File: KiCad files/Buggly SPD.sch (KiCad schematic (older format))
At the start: 6 parts, among them J1 Conn_01x07, J2 Conn_01x05, J3 Conn_01x08, J4 Conn_01x02, J5 Conn_02x03_Odd_Even, J6 Conn_01x02

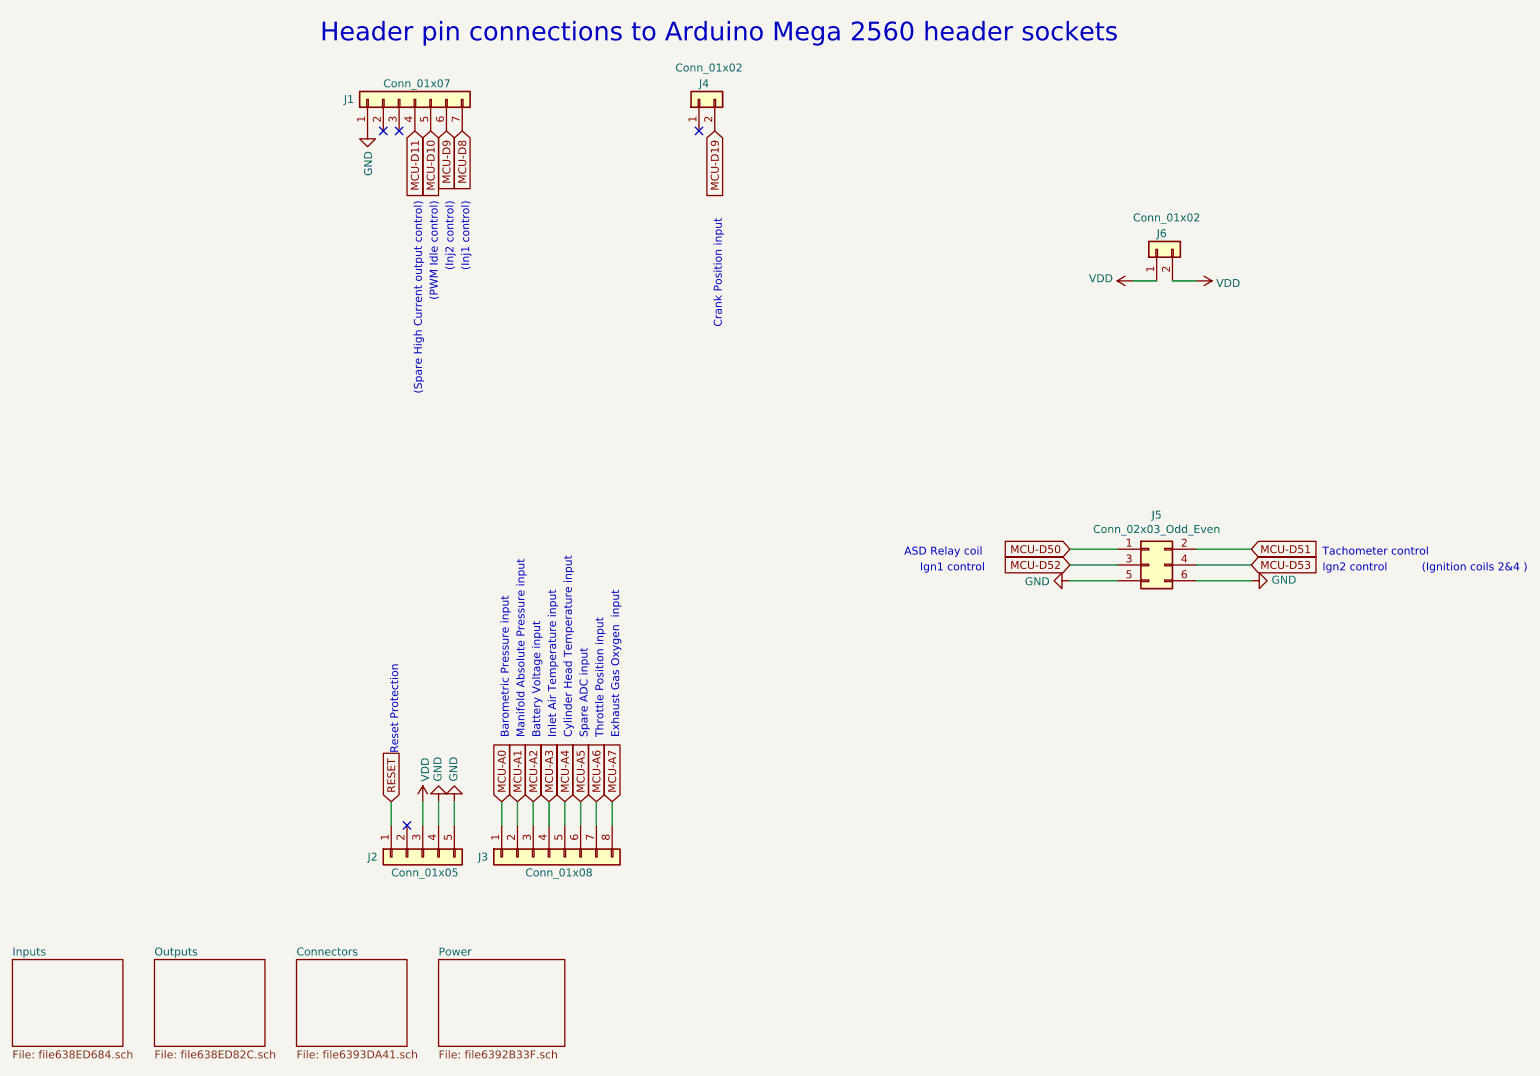
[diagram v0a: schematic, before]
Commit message: Add files via upload
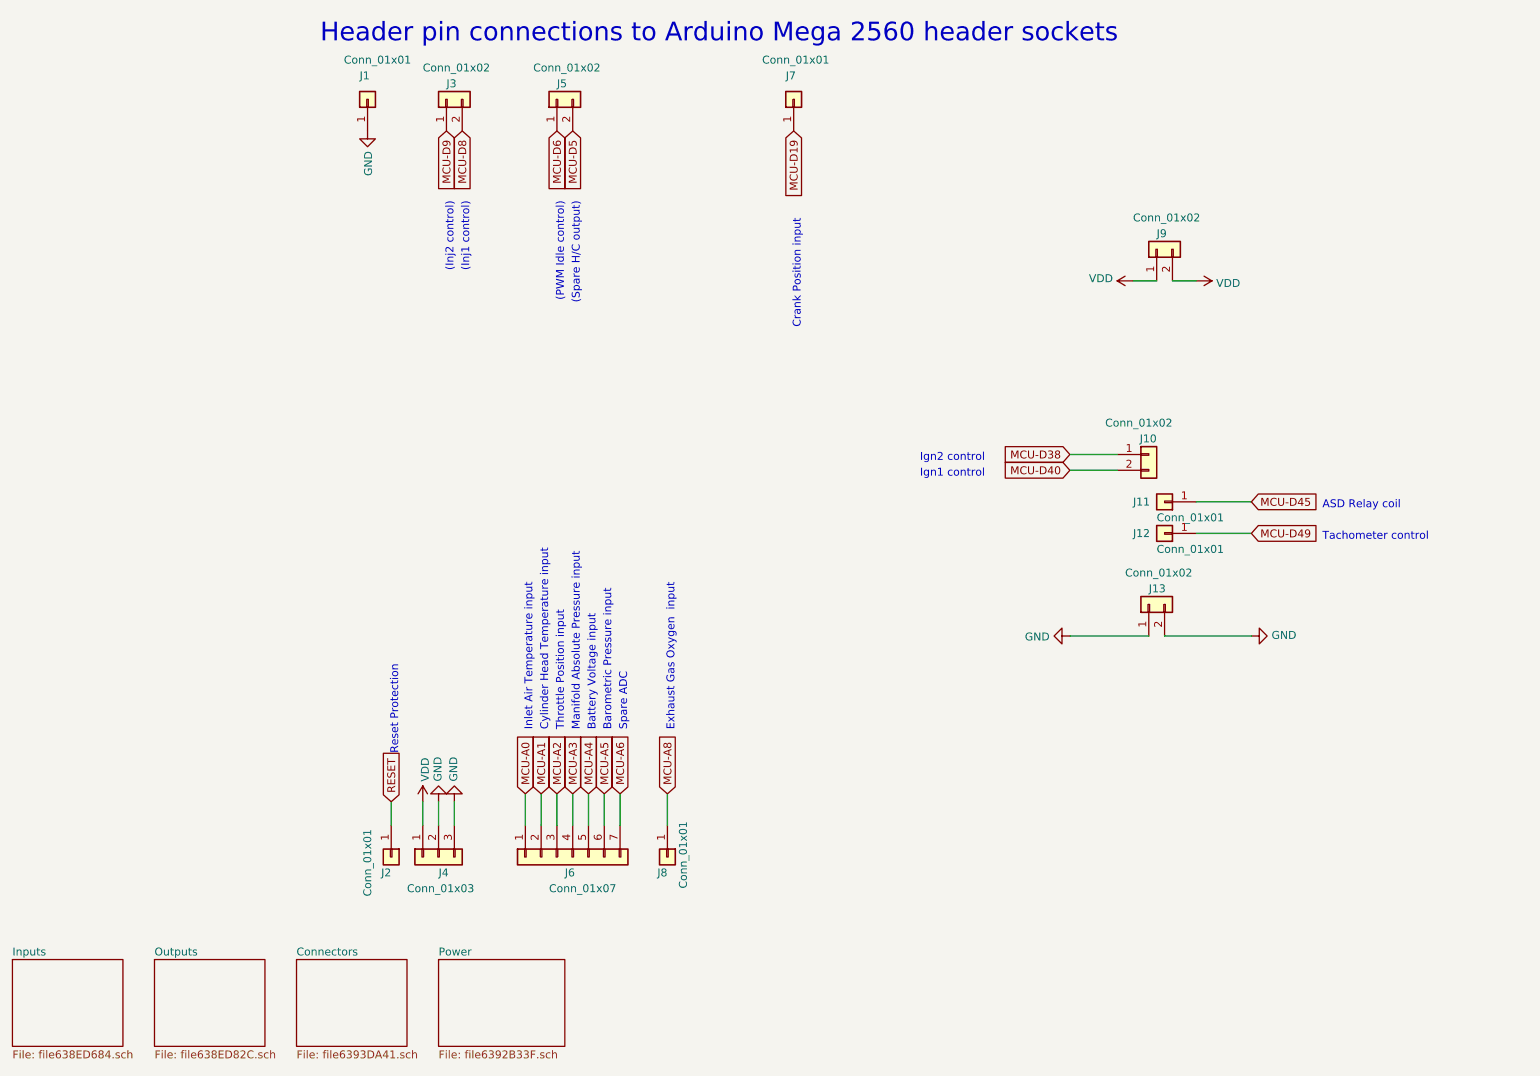
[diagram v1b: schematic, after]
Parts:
- removed J1: Conn_01x07, Connector_PinHeader_2.54mm:PinHeader_1x07_P2.54mm_Vertical, symbol Connector_Generic:Conn_01x07
- removed J2: Conn_01x05, Connector_PinHeader_2.54mm:PinHeader_1x05_P2.54mm_Vertical, symbol Connector_Generic:Conn_01x05
- removed J3: Conn_01x08, Connector_PinHeader_2.54mm:PinHeader_1x08_P2.54mm_Vertical, symbol Connector_Generic:Conn_01x08
- removed J4: Conn_01x02, Connector_PinHeader_2.54mm:PinHeader_1x02_P2.54mm_Vertical, symbol Connector_Generic:Conn_01x02
- removed J5: Conn_02x03_Odd_Even, Connector_PinHeader_2.54mm:PinHeader_2x03_P2.54mm_Vertical, symbol Connector_Generic:Conn_02x03_Odd_Even
- added J1, J11, J12, J2, J7, J8: Conn_01x01, Connector_PinHeader_2.54mm:PinHeader_1x01_P2.54mm_Vertical, symbol Connector_Generic:Conn_01x01
- added J10, J13, J3, J5: Conn_01x02, Connector_PinHeader_2.54mm:PinHeader_1x02_P2.54mm_Vertical, symbol Connector_Generic:Conn_01x02
- added J4: Conn_01x03, Connector_PinHeader_2.54mm:PinHeader_1x03_P2.54mm_Vertical, symbol Connector_Generic:Conn_01x03
- added J6: Conn_01x07, Connector_PinHeader_2.54mm:PinHeader_1x07_P2.54mm_Vertical, symbol Connector_Generic:Conn_01x07
- renumbered J6 to J9
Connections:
- net GND: now also J1.1 (Pin_1), J13.1 (Pin_1), J13.2 (Pin_2), J4.2 (Pin_2), J4.3 (Pin_3)
- net MCU-A0: now also J6.1 (Pin_1)
- net MCU-A1: now also J6.2 (Pin_2)
- net MCU-A2: now also J6.3 (Pin_3)
- net MCU-A3: now also J6.4 (Pin_4)
- net MCU-A4: now also J6.5 (Pin_5)
- net MCU-A5: now also J6.6 (Pin_6)
- net MCU-A6: now also J6.7 (Pin_7)
- net MCU-D19: now also J7.1 (Pin_1)
- net MCU-D8: now also J3.2 (Pin_2)
- net MCU-D9: now also J3.1 (Pin_1)
- net RESET: now also J2.1 (Pin_1)
- net VDD: now also J4.1 (Pin_1)
- new net MCU-A8: J8.1 (Pin_1)
- new net MCU-D38: J10.1 (Pin_1)
- new net MCU-D40: J10.2 (Pin_2)
- new net MCU-D45: J11.1 (Pin_1)
- new net MCU-D49: J12.1 (Pin_1)
- new net MCU-D5: J5.2 (Pin_2)
- new net MCU-D6: J5.1 (Pin_1)
- no-connect marks 4 -> 0
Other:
- note added: "(Spare H/C output)"
- note added: "Spare ADC"
- note removed: "(Ignition coils 2&4 )"
- note removed: "(Spare High Current output control)"
- note removed: "Spare ADC input"

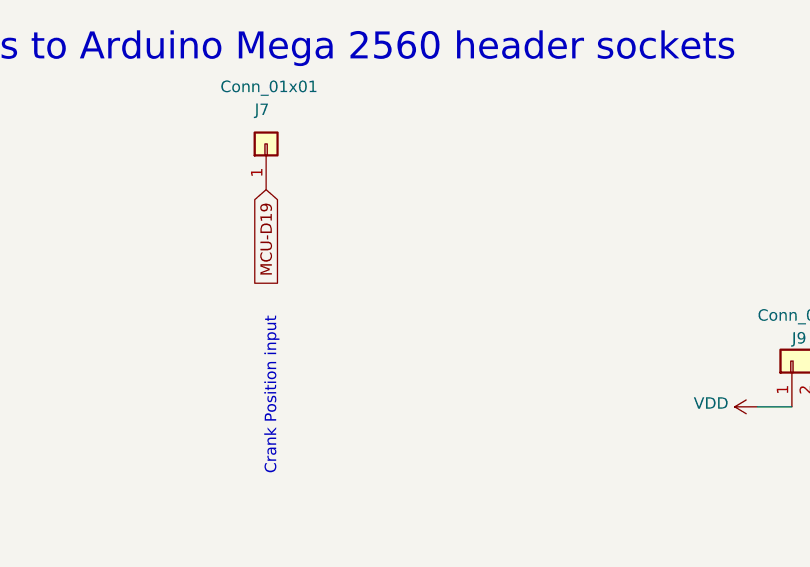
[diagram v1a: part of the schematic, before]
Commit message: Add files via upload
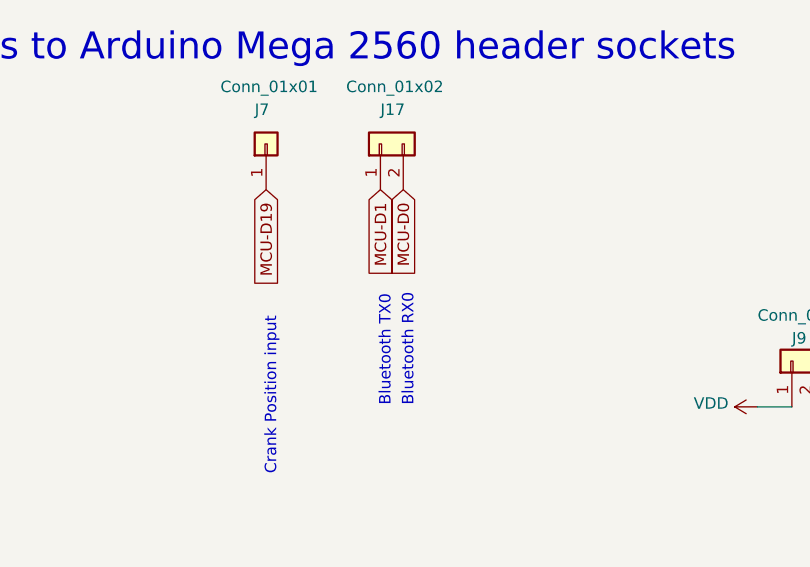
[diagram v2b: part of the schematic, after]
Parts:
- added J17: Conn_01x02, Connector_PinHeader_2.54mm:PinHeader_1x02_P2.54mm_Vertical, symbol Connector_Generic:Conn_01x02
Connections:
- new net MCU-D0: J17.2 (Pin_2)
- new net MCU-D1: J17.1 (Pin_1)
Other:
- note added: "Bluetooth RX0"
- note added: "Bluetooth TX0"
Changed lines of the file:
@@
 Wire Wire Line
 	4500 6000 4500 6200
+$Comp
+L Connector_Generic:Conn_01x02 J17
+U 1 1 63BC3131
+P 6100 1600
+F 0 "J17" V 6250 1600 50  0000 R CNN
+F 1 "Conn_01x02" V 6350 1750 50  0000 R CNN
+F 2 "Connector_PinHeader_2.54mm:PinHeader_1x02_P2.54mm_Vertical" H 6100 1600 50  0001 C CNN
+F 3 "~" H 6100 1600 50  0001 C CNN
+	1    6100 1600
+	0    -1   -1   0
+$EndComp
+Text GLabel 6200 1800 3    50   Input ~ 0
+MCU-D0
+Text GLabel 6100 1800 3    50   Input ~ 0
+MCU-D1
+Text Notes 6250 2750 1    50   ~ 0
+Bluetooth RX0
+Text Notes 6150 2750 1    50   ~ 0
+Bluetooth TX0
 $EndSCHEMATC
